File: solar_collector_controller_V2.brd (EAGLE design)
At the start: 49.5 x 50 mm, 32 parts, among them IC1 REG1117, J1 POWER, T1 BC337, X1 GND D2 VCC, X2 GND D9 VCC, X3 GND A3 VCC, X4 VCC A4 A5 GND, X5 GND A1 A2 VCC, X6 A7 A6

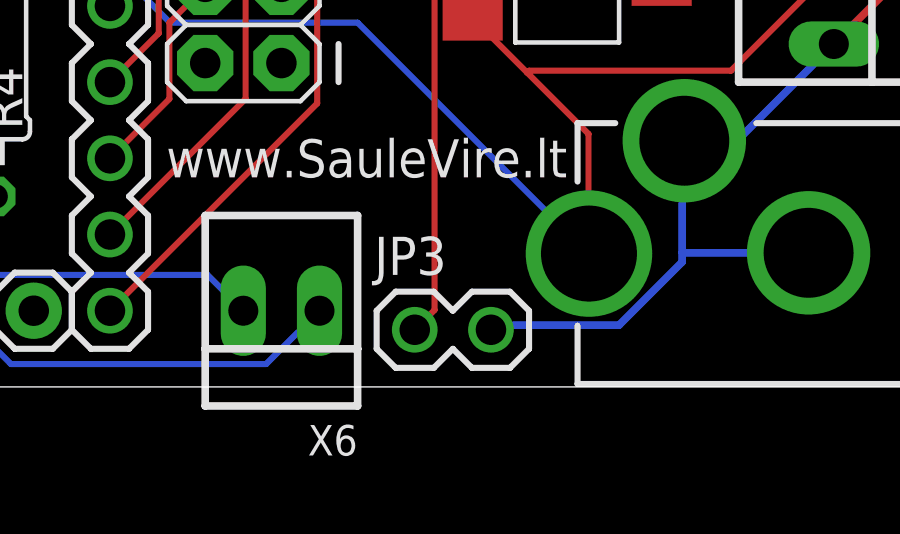
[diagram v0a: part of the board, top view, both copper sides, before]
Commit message: Finito, paruo6ta siuntimui
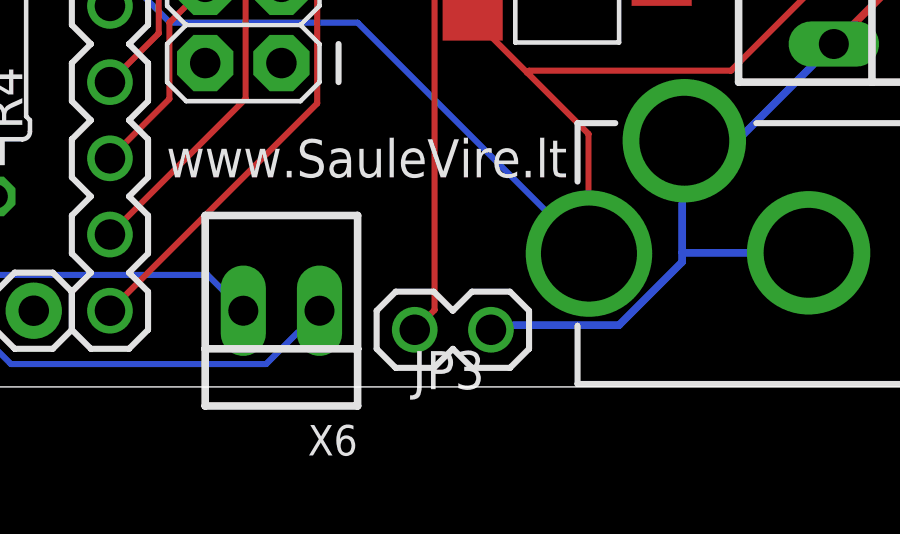
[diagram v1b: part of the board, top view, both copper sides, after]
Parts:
- JP3: value (none) -> GND 3.3V
- X1: value GND D2 VCC -> VCC D2 GND
- X2: value GND D9 VCC -> VCC D9 GND
- X3: value GND A3 VCC -> VCC A3 GND
- X4: value VCC A4 A5 GND -> GND A5 A4 VCC
- X5: value GND A1 A2 VCC -> VCC A2 A1 GND
- X6: value A7 A6 -> A6 A7
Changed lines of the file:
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@@
 <element name="LCD1602" library="Connector_seedstudio" package="16P-2.54" value="" x="2.54" y="43.815" rot="R270"/>
 <element name="R5" library="resistor" package="RTRIM64W" value="10k" x="10.16" y="41.275" rot="R270"/>
-<element name="X1" library="con-molex" package="22-23-2031" value="GND D2 VCC" x="29.21" y="46.99" smashed="yes">
+<element name="X1" library="con-molex" package="22-23-2031" value="VCC D2 GND" x="29.21" y="46.99" smashed="yes">
 <attribute name="OC_NEWARK" value="30C0862" x="29.21" y="46.99" size="1.778" layer="27" display="off"/>
 <attribute name="MPN" value="22-23-2031" x="29.21" y="46.99" size="1.778" layer="27" display="off"/>
@@
 <attribute name="OC_FARNELL" value="1462950" x="29.21" y="46.99" size="1.778" layer="27" display="off"/>
 <attribute name="NAME" x="25.4" y="50.8" size="1.016" layer="25" ratio="10"/>
-<attribute name="VALUE" x="26.035" y="48.895" size="0.8" layer="27" ratio="10"/>
+<attribute name="VALUE" x="32.385" y="48.895" size="0.8" layer="28" ratio="10" rot="MR0"/>
 </element>
-<element name="X2" library="con-molex" package="22-23-2031" value="GND D9 VCC" x="19.05" y="46.99" smashed="yes">
+<element name="X2" library="con-molex" package="22-23-2031" value="VCC D9 GND" x="19.05" y="46.99" smashed="yes">
 <attribute name="OC_NEWARK" value="30C0862" x="19.05" y="46.99" size="1.778" layer="27" display="off"/>
 <attribute name="MPN" value="22-23-2031" x="19.05" y="46.99" size="1.778" layer="27" display="off"/>
@@
 <attribute name="OC_FARNELL" value="1462950" x="19.05" y="46.99" size="1.778" layer="27" display="off"/>
 <attribute name="NAME" x="15.24" y="50.8" size="1.016" layer="25" ratio="10"/>
-<attribute name="VALUE" x="15.875" y="48.895" size="0.8" layer="27" ratio="10"/>
+<attribute name="VALUE" x="22.225" y="48.895" size="0.8" layer="28" ratio="10" rot="MR0"/>
 </element>
-<element name="X3" library="con-molex" package="22-23-2031" value="GND A3 VCC" x="8.89" y="46.99" smashed="yes">
+<element name="X3" library="con-molex" package="22-23-2031" value="VCC A3 GND" x="8.89" y="46.99" smashed="yes">
 <attribute name="OC_NEWARK" value="30C0862" x="8.89" y="46.99" size="1.778" layer="27" display="off"/>
 <attribute name="MPN" value="22-23-2031" x="8.89" y="46.99" size="1.778" layer="27" display="off"/>
@@
 <attribute name="OC_FARNELL" value="1462950" x="8.89" y="46.99" size="1.778" layer="27" display="off"/>
 <attribute name="NAME" x="5.08" y="50.8" size="1.016" layer="25" ratio="10"/>
-<attribute name="VALUE" x="5.715" y="48.895" size="0.8" layer="27" ratio="10"/>
+<attribute name="VALUE" x="12.065" y="48.895" size="0.8" layer="28" ratio="10" rot="MR0"/>
 </element>
 <element name="S1" library="switch-omron" package="B3F-10XX" value="Right" x="38.735" y="39.37" smashed="yes" rot="R180">
@@
 <attribute name="OC_FARNELL" value="176432" x="38.735" y="31.115" size="1.778" layer="27" rot="R270" display="off"/>
 </element>
-<element name="X5" library="con-molex" package="22-23-2041" value="GND A1   A2 VCC" x="40.64" y="46.99" smashed="yes">
+<element name="X5" library="con-molex" package="22-23-2041" value="VCC A2   A1 GND" x="40.64" y="46.99" smashed="yes">
 <attribute name="OC_NEWARK" value="38C0355" x="40.64" y="46.99" size="1.778" layer="27" display="off"/>
 <attribute name="MPN" value="22-23-2041" x="40.64" y="46.99" size="1.778" layer="27" display="off"/>
@@
 <attribute name="OC_FARNELL" value="1462920" x="40.64" y="46.99" size="1.778" layer="27" display="off"/>
 <attribute name="NAME" x="35.56" y="50.8" size="1.016" layer="25" ratio="10"/>
-<attribute name="VALUE" x="36.195" y="48.895" size="0.8" layer="27" ratio="10"/>
+<attribute name="VALUE" x="36.195" y="49.53" size="0.8" layer="28" ratio="10" rot="MR180"/>
 </element>
 <element name="T1" library="transistor" package="TO92" value="BC337" x="6.35" y="36.83" smashed="yes" rot="R180">
 <attribute name="NAME" x="3.175" y="36.195" size="1.27" layer="25" ratio="10" rot="R180"/>
-<attribute name="VALUE" x="3.175" y="38.1" size="1.27" layer="27" ratio="10" rot="R180"/>
+<attribute name="VALUE" x="13.97" y="38.735" size="1.27" layer="27" ratio="10" rot="R180"/>
 </element>
 <element name="R6" library="resistor" package="0207/10" value="3k3" x="31.75" y="21.59" smashed="yes" rot="R90">
@@
 <attribute name="VALUE" x="33.528" y="18.034" size="1.27" layer="27" ratio="10" rot="R270"/>
 </element>
-<element name="X4" library="con-molex" package="22-23-2041" value="VCC A4 A5 GND" x="46.99" y="15.24" smashed="yes" rot="R270">
+<element name="X4" library="con-molex" package="22-23-2041" value="GND A5 A4 VCC" x="46.99" y="15.24" smashed="yes" rot="R270">
 <attribute name="OC_NEWARK" value="38C0355" x="46.99" y="15.24" size="1.778" layer="27" rot="R270" display="off"/>
 <attribute name="MPN" value="22-23-2041" x="46.99" y="15.24" size="1.778" layer="27" rot="R270" display="off"/>
@@
 <attribute name="OC_FARNELL" value="1462920" x="46.99" y="15.24" size="1.778" layer="27" rot="R270" display="off"/>
 <attribute name="NAME" x="48.895" y="14.605" size="1.016" layer="25" ratio="10" rot="R270"/>
-<attribute name="VALUE" x="46.99" y="20.32" size="1.016" layer="27" ratio="10" rot="R270"/>
+<attribute name="VALUE" x="46.99" y="20.32" size="1.016" layer="28" ratio="10" rot="MR270"/>
 </element>
-<element name="X6" library="con-molex" package="22-23-2021" value="   A7 A6" x="28.575" y="2.54" smashed="yes" rot="R180">
+<element name="X6" library="con-molex" package="22-23-2021" value="   A6 A7" x="28.575" y="2.54" smashed="yes" rot="R180">
 <attribute name="OC_NEWARK" value="25C3832" x="28.575" y="2.54" size="1.778" layer="27" rot="R180" display="off"/>
 <attribute name="MPN" value="22-23-2021" x="28.575" y="2.54" size="1.778" layer="27" rot="R180" display="off"/>
@@
 <attribute name="OC_FARNELL" value="1462926" x="28.575" y="2.54" size="1.778" layer="27" rot="R180" display="off"/>
 <attribute name="NAME" x="31.115" y="-1.27" size="1.016" layer="25" ratio="10" rot="R180"/>
-<attribute name="VALUE" x="30.48" y="5.08" size="1.016" layer="27" ratio="10" rot="R180"/>
+<attribute name="VALUE" x="26.67" y="5.08" size="1.016" layer="28" ratio="10" rot="MR180"/>
 </element>
-<element name="JP3" library="SparkFun" package="1X02" value="" x="33.02" y="1.905"/>
+<element name="JP3" library="SparkFun" package="1X02" value="GND 3.3V" x="33.02" y="1.905" smashed="yes">
+<attribute name="NAME" x="32.9438" y="-0.0762" size="1.27" layer="25" ratio="10"/>
+<attribute name="VALUE" x="37.465" y="3.175" size="1" layer="28" rot="MR0"/>
+</element>
 </elements>
 <signals>
